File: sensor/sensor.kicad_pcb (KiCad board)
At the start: 2 copper layers, 57.1 x 76.2 mm, 9 parts, among them T1 DS18B20, T2 DS18B20, U1 DHT22, U2 SSCDRNN015PASA5

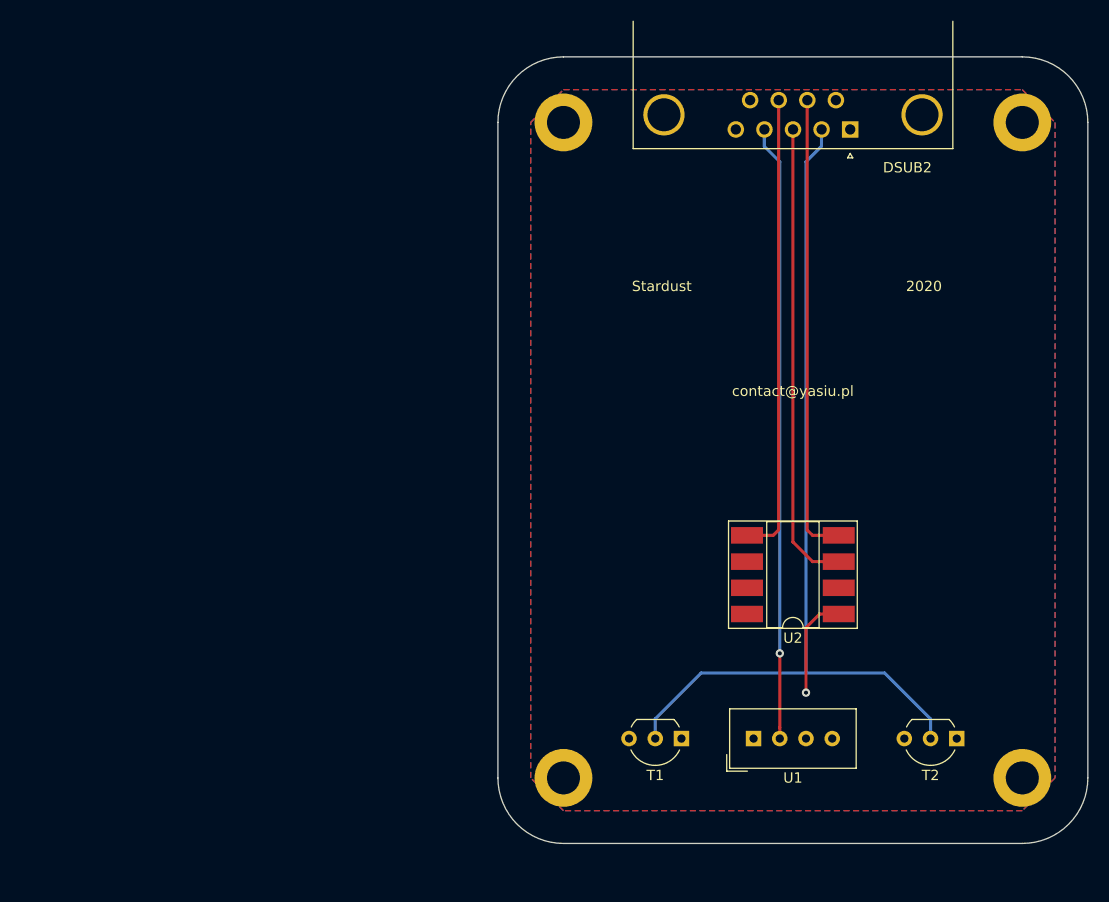
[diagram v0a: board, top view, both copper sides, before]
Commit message: WIP sensor PCB
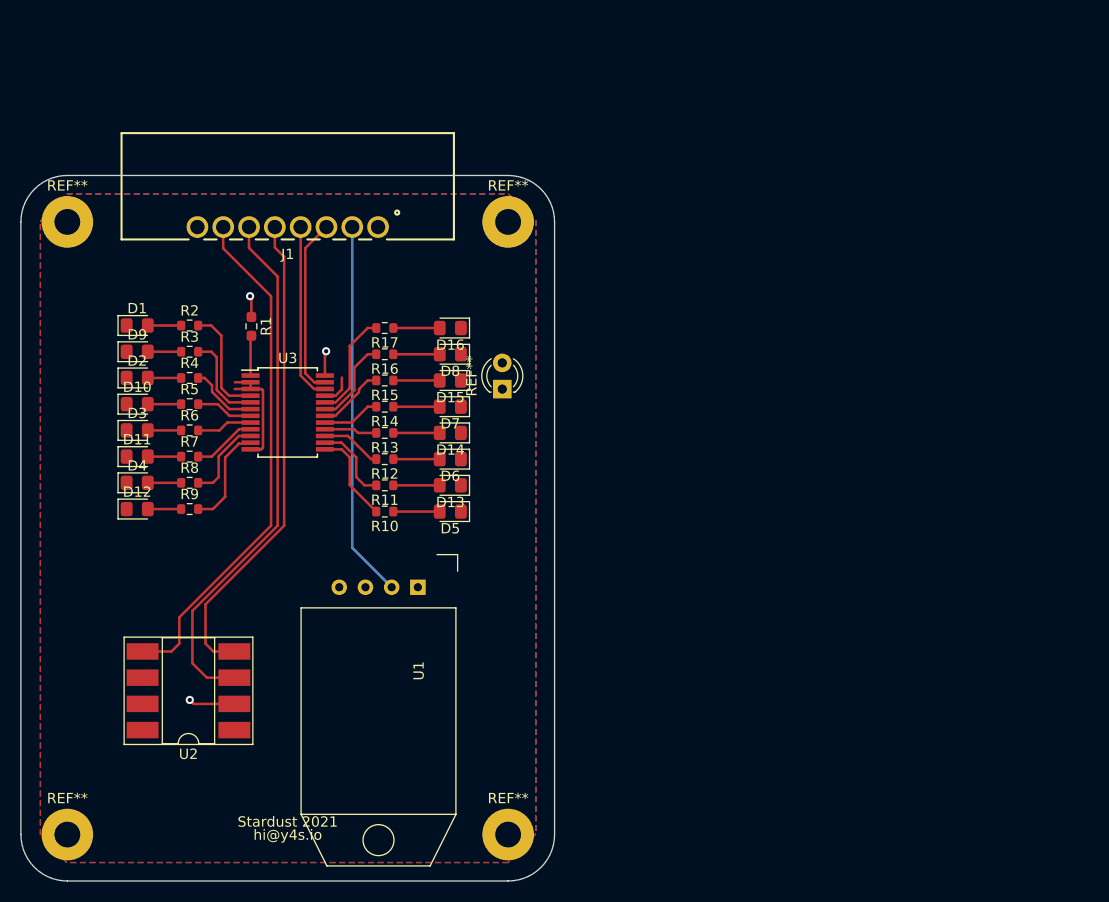
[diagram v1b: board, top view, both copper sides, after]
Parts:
- removed DSUB2: DB9_Male, Connector_Dsub:DSUB-9_Male_Horizontal_P2.77x2.84mm_EdgePinOffset7.70mm_Housed_MountingHolesOffset9.12mm
- removed the REF** at (228.6, 114.3)
- removed the REF** at (184.2, 114.3)
- removed the REF** at (184.2, 50.8)
- removed the REF** at (228.6, 50.8)
- removed T1, T2: DS18B20, Package_TO_SOT_THT:TO-92_Inline_Wide
- added D1: LED, LED_SMD:LED_0805_2012Metric_Pad1.15x1.40mm_HandSolder, F.Cu at (142.9, 70.5)
- added D10: LED, LED_SMD:LED_0805_2012Metric_Pad1.15x1.40mm_HandSolder, F.Cu at (142.9, 78.1)
- added D11: LED, LED_SMD:LED_0805_2012Metric_Pad1.15x1.40mm_HandSolder, F.Cu at (142.9, 83.2)
- added D12: LED, LED_SMD:LED_0805_2012Metric_Pad1.15x1.40mm_HandSolder, F.Cu at (142.9, 88.3)
- added D13: LED, LED_SMD:LED_0805_2012Metric_Pad1.15x1.40mm_HandSolder, F.Cu at (173.2, 86.0)
- added D14: LED, LED_SMD:LED_0805_2012Metric_Pad1.15x1.40mm_HandSolder, F.Cu at (173.2, 80.9)
- added D15: LED, LED_SMD:LED_0805_2012Metric_Pad1.15x1.40mm_HandSolder, F.Cu at (173.2, 75.8)
- added D16: LED, LED_SMD:LED_0805_2012Metric_Pad1.15x1.40mm_HandSolder, F.Cu at (173.2, 70.7)
- added D2: LED, LED_SMD:LED_0805_2012Metric_Pad1.15x1.40mm_HandSolder, F.Cu at (142.9, 75.6)
- added D3: LED, LED_SMD:LED_0805_2012Metric_Pad1.15x1.40mm_HandSolder, F.Cu at (142.9, 80.6)
- added D4: LED, LED_SMD:LED_0805_2012Metric_Pad1.15x1.40mm_HandSolder, F.Cu at (142.9, 85.7)
- added D5: LED, LED_SMD:LED_0805_2012Metric_Pad1.15x1.40mm_HandSolder, F.Cu at (173.2, 88.5)
- added D6: LED, LED_SMD:LED_0805_2012Metric_Pad1.15x1.40mm_HandSolder, F.Cu at (173.2, 83.4)
- added D7: LED, LED_SMD:LED_0805_2012Metric_Pad1.15x1.40mm_HandSolder, F.Cu at (173.2, 78.3)
- added D8: LED, LED_SMD:LED_0805_2012Metric_Pad1.15x1.40mm_HandSolder, F.Cu at (173.2, 73.3)
- added D9: LED, LED_SMD:LED_0805_2012Metric_Pad1.15x1.40mm_HandSolder, F.Cu at (142.9, 73.0)
- added J1: Conn_01x08_Female, Stardust:691382040008, F.Cu at (157.4, 60.9)
- added R1: R10k, Resistor_SMD:R_0603_1608Metric_Pad0.98x0.95mm_HandSolder, F.Cu at (153.9, 70.6)
- added R10: R330, Resistor_SMD:R_0603_1608Metric, F.Cu at (166.8, 88.5)
- added R11: R330, Resistor_SMD:R_0603_1608Metric, F.Cu at (166.8, 86.0)
- added R12: R330, Resistor_SMD:R_0603_1608Metric, F.Cu at (166.8, 83.4)
- added R13: R330, Resistor_SMD:R_0603_1608Metric, F.Cu at (166.8, 80.9)
- added R14: R330, Resistor_SMD:R_0603_1608Metric, F.Cu at (166.8, 78.3)
- added R15: R330, Resistor_SMD:R_0603_1608Metric, F.Cu at (166.8, 75.8)
- added R16: R330, Resistor_SMD:R_0603_1608Metric, F.Cu at (166.8, 73.3)
- added R17: R330, Resistor_SMD:R_0603_1608Metric, F.Cu at (166.8, 70.7)
- added R2: R330, Resistor_SMD:R_0603_1608Metric, F.Cu at (147.9, 70.5)
- added R3: R330, Resistor_SMD:R_0603_1608Metric, F.Cu at (147.9, 73.0)
- added R4: R330, Resistor_SMD:R_0603_1608Metric, F.Cu at (147.9, 75.6)
- added R5: R330, Resistor_SMD:R_0603_1608Metric, F.Cu at (147.9, 78.1)
- added R6: R330, Resistor_SMD:R_0603_1608Metric, F.Cu at (147.9, 80.6)
- added R7: R330, Resistor_SMD:R_0603_1608Metric, F.Cu at (147.9, 83.2)
- added R8: R330, Resistor_SMD:R_0603_1608Metric, F.Cu at (147.9, 85.7)
- added R9: R330, Resistor_SMD:R_0603_1608Metric, F.Cu at (147.9, 88.3)
- added REF**: LED_D3.0mm, LED_THT:LED_D3.0mm, F.Cu at (178.2, 76.6)
- added REF**: MountingHole_2.5mm_Pad, MountingHole:MountingHole_2.5mm_Pad, F.Cu at (136.1, 119.8)
- added REF**: MountingHole_2.5mm_Pad, MountingHole:MountingHole_2.5mm_Pad, F.Cu at (178.8, 119.8)
- added REF**: MountingHole_2.5mm_Pad, MountingHole:MountingHole_2.5mm_Pad, F.Cu at (178.8, 60.4)
- added REF**: MountingHole_2.5mm_Pad, MountingHole:MountingHole_2.5mm_Pad, F.Cu at (136.1, 60.4)
- added U3: TCA9555DBR, Package_SO:SSOP-24_5.3x8.2mm_P0.65mm, F.Cu at (157.4, 78.9)
- U1: footprint Sensor:Aosong_DHT11_5.5x12.0_P2.54mm -> Stardust:DHT22_15.0x25.0_P2.54mm_Horizontal
- moved U2 59.6 mm to (147.8, 105.9)
- moved U1 35.7 mm to (170.0, 95.8), turned to 270 degrees
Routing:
- net 1Wire: track 87.4 -> 0.00 mm
- net DHT22: track 59.6 -> 36.5 mm, vias 1 -> 0
- net SDA: track 0.00 -> 17.3 mm
- net SCL: track 0.00 -> 17.3 mm
- net Net-(R2-Pad2): track 0.00 -> 10.9 mm
- net Net-(R17-Pad2): track 0.00 -> 10.4 mm
- net Net-(R9-Pad2): track 0.00 -> 10.0 mm
- net Net-(R10-Pad2): track 0.00 -> 9.04 mm
- net Net-(R3-Pad2): track 0.00 -> 8.97 mm
- net +5V: track 0.00 -> 8.94 mm, vias 0 -> 3
- net Net-(R16-Pad2): track 0.00 -> 8.46 mm
- net Net-(R8-Pad2): track 0.00 -> 8.14 mm
- net Net-(R11-Pad2): track 0.00 -> 7.81 mm
- net Net-(R4-Pad2): track 0.00 -> 6.70 mm
- net Net-(R15-Pad2): track 0.00 -> 6.56 mm
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- added copper zone on B.Cu, net +5V
- added copper zone on F.Cu, net GND
- removed copper zone on F.Cu, net +5V
- removed copper zone on B.Cu, net GND
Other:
- board size 57.1 x 76.2 mm -> 51.7 x 68.4 mm
- board text added: "Stardust 2021"
- board text added: "hi@y4s.io"
- board text removed: "2020"
- board text removed: "Stardust"
- board text removed: "contact@yasiu.pl"
